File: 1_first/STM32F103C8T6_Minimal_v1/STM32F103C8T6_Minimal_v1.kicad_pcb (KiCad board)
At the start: 4 copper layers, 34 parts, among them J1 Conn_01x06, J2 USB_B_Micro, SW1 SW_SPDT, SW2 SW_Push, SW3 SW_Push, U1 AMS1117-3.3, U2 STM32F103C8Tx, U3 USBLC6-2SC6, Y1 8MHz

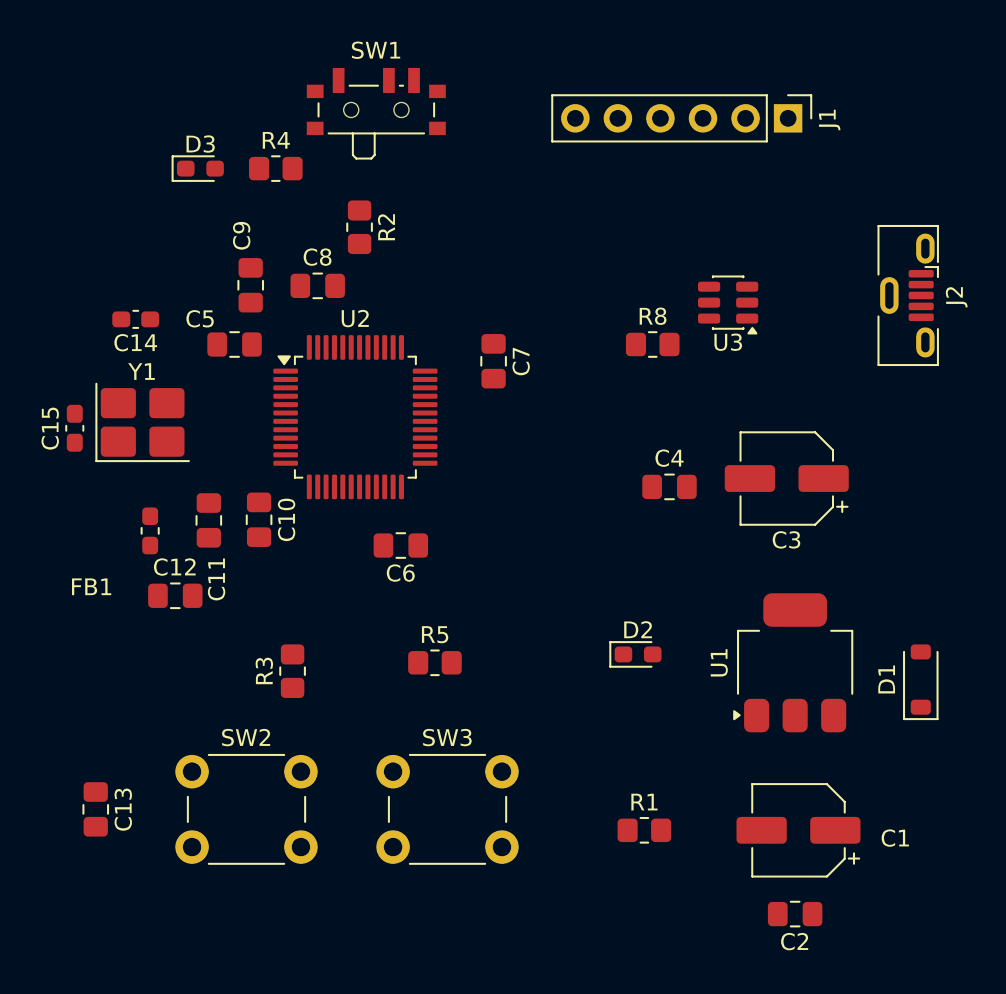
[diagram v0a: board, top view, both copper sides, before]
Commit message: Board cut
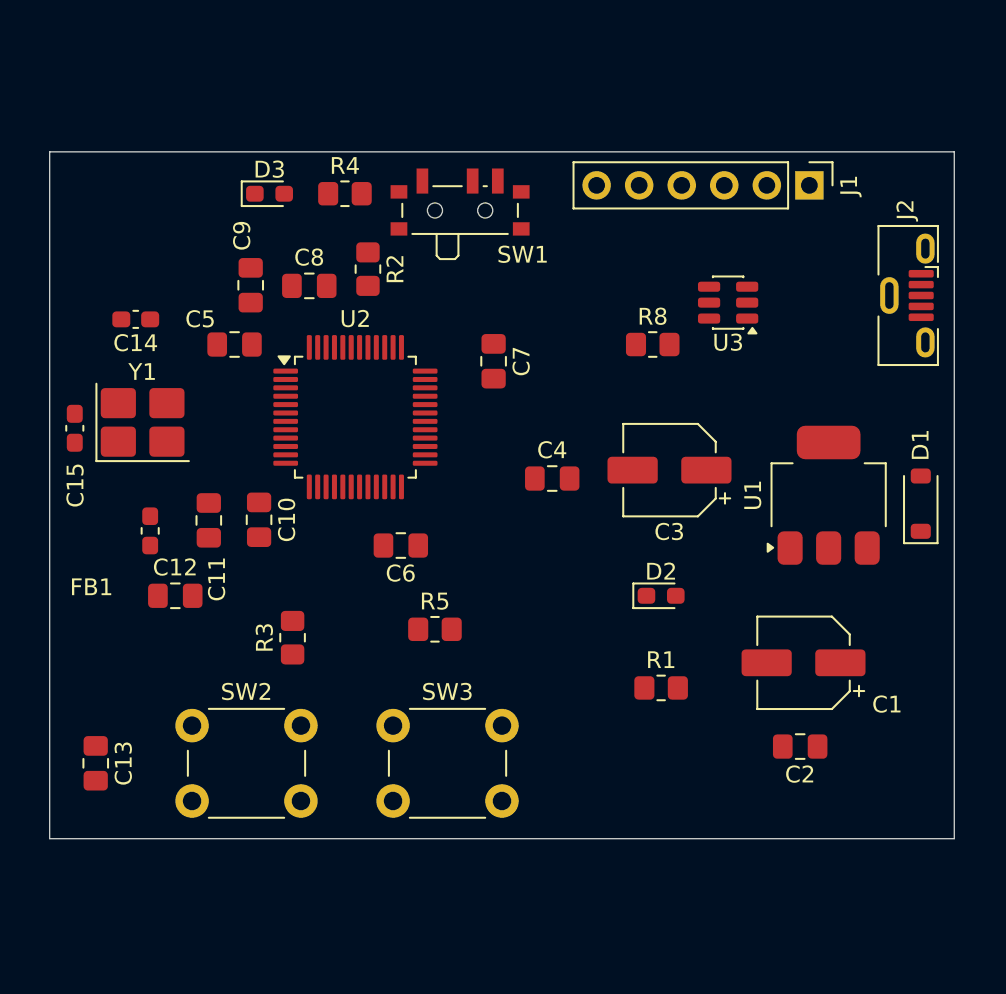
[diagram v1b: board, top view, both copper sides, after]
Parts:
- moved D1 10.5 mm to (154.0, 100.0)
- moved U1 10.2 mm to (148.5, 99.5)
- moved C1 10.0 mm to (147.0, 109.5)
- moved C2 10.0 mm to (146.8, 114.5)
- moved R1 8.56 mm to (138.5, 111.0)
- moved SW1 7.81 mm to (126.5, 82.2)
- moved C3 7.02 mm to (139.0, 98.0)
- moved C4 7.02 mm to (132.0, 98.5)
- moved D3 4.39 mm to (115.1, 81.5)
- moved R4 4.39 mm to (119.6, 81.5)
- moved J1 4.20 mm to (147.3, 81.0)
- moved D2 3.76 mm to (138.5, 105.5)
- moved C13 2.75 mm to (104.8, 115.5)
- moved SW2 2.75 mm to (110.5, 113.2)
- moved SW3 2.75 mm to (122.5, 113.2)
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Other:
- board outline added: 54 x 41 mm
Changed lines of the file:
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@@
 	(footprint "Capacitor_SMD:CP_Elec_5x5.3"
 		(layer "F.Cu")
-		(at 146.7 119.5 180)
+		(at 147 109.5 180)
 		(descr "SMD capacitor, aluminum electrolytic, Nichicon, 5.0x5.3mm")
 		(tags "capacitor electrolytic")
 		(property "Reference" "C1"
-			(at -5.8 -0.5 0)
+			(at -5 -2.5 0)
 			(layer "F.SilkS")
 			(effects
@@
 	(footprint "Connector_PinHeader_2.54mm:PinHeader_1x06_P2.54mm_Vertical"
 		(layer "F.Cu")
-		(at 146.08 77 -90)
+		(at 147.35 81 -90)
 		(descr "Through hole straight pin header, 1x06, 2.54mm pitch, single row")
 		(tags "Through hole pin header THT 1x06 2.54mm single row")
@@
 		)
 		(property "Value" "Conn_01x06"
-			(at 0 15.08 90)
+			(at 2.35 7.4 180)
 			(layer "F.Fab")
 			(effects
@@
 	(footprint "Capacitor_SMD:CP_Elec_5x5.3"
 		(layer "F.Cu")
-		(at 146 98.5 180)
+		(at 139 98 180)
 		(descr "SMD capacitor, aluminum electrolytic, Nichicon, 5.0x5.3mm")
 		(tags "capacitor electrolytic")
@@
 	(footprint "Button_Switch_THT:SW_PUSH_6mm_H5mm"
 		(layer "F.Cu")
-		(at 122.5 116)
+		(at 122.5 113.25)
 		(descr "tactile push button, 6x6mm e.g. PHAP33xx series, height=5mm")
 		(tags "tact sw push 6mm")
@@
 		)
 		(property "Value" "SW_Push"
-			(at 3.75 6.7 0)
+			(at 11.35 2.5 0)
 			(layer "F.Fab")
 			(effects
@@
 	(footprint "Button_Switch_THT:SW_PUSH_6mm_H5mm"
 		(layer "F.Cu")
-		(at 110.5 116)
+		(at 110.5 113.25)
 		(descr "tactile push button, 6x6mm e.g. PHAP33xx series, height=5mm")
 		(tags "tact sw push 6mm")
@@
 		)
 		(property "Value" "SW_Push"
-			(at 3.75 6.7 0)
+			(at -4.75 5.45 0)
 			(layer "F.Fab")
 			(effects
@@
 	(footprint "Resistor_SMD:R_0805_2012Metric_Pad1.20x1.40mm_HandSolder"
 		(layer "F.Cu")
-		(at 115.5 80)
+		(at 119.625 81.5)
 		(descr "Resistor SMD 0805 (2012 Metric), square (rectangular) end terminal, IPC-7351 nominal with elongated pad for handsoldering. (Body size source: IPC-SM-782 page 72, https://www.pcb-3d.com/wordpress/wp-content/uploads/ipc-sm-782a_amendment_1_and_2.pdf)")
 		(tags "resistor handsolder")
@@
 	(footprint "Resistor_SMD:R_0805_2012Metric_Pad1.20x1.40mm_HandSolder"
 		(layer "F.Cu")
-		(at 120.5 83.5 -90)
+		(at 121 86 -90)
 		(descr "Resistor SMD 0805 (2012 Metric), square (rectangular) end terminal, IPC-7351 nominal with elongated pad for handsoldering. (Body size source: IPC-SM-782 page 72, https://www.pcb-3d.com/wordpress/wp-content/uploads/ipc-sm-782a_amendment_1_and_2.pdf)")
 		(tags "resistor handsolder")
@@
 	(footprint "LED_SMD:LED_0603_1608Metric_Pad1.05x0.95mm_HandSolder"
 		(layer "F.Cu")
-		(at 111 80)
+		(at 115.125 81.5)
 		(descr "LED SMD 0603 (1608 Metric), square (rectangular) end terminal, IPC-7351 nominal, (Body size source: http://www.tortai-tech.com/upload/download/2011102023233369053.pdf)")
 		(tags "LED handsolder")
@@
 	(footprint "Resistor_SMD:R_0805_2012Metric_Pad1.20x1.40mm_HandSolder"
 		(layer "F.Cu")
-		(at 125 109.5)
+		(at 125 107.5)
 		(descr "Resistor SMD 0805 (2012 Metric), square (rectangular) end terminal, IPC-7351 nominal with elongated pad for handsoldering. (Body size source: IPC-SM-782 page 72, https://www.pcb-3d.com/wordpress/wp-content/uploads/ipc-sm-782a_amendment_1_and_2.pdf)")
 		(tags "resistor handsolder")
@@
 	(footprint "LED_SMD:LED_0603_1608Metric_Pad1.05x0.95mm_HandSolder"
 		(layer "F.Cu")
-		(at 137.125 109)
+		(at 138.5 105.5)
 		(descr "LED SMD 0603 (1608 Metric), square (rectangular) end terminal, IPC-7351 nominal, (Body size source: http://www.tortai-tech.com/upload/download/2011102023233369053.pdf)")
 		(tags "LED handsolder")
@@
 	(footprint "Diode_SMD:D_SOD-123"
 		(layer "F.Cu")
-		(at 154 110.5 90)
+		(at 154 100 90)
 		(descr "SOD-123")
 		(tags "SOD-123")
 		(property "Reference" "D1"
-			(at 0 -2 90)
+			(at 3.5 0 90)
 			(layer "F.SilkS")
 			(effects
@@
 		)
 		(property "Value" "D_Schottky"
-			(at 0 2.1 90)
+			(at -6.5 0 270)
 			(layer "F.Fab")
 			(effects
@@
 		)
 		(fp_text user "${REFERENCE}"
-			(at 0 -2 90)
+			(at 3.5 0 90)
 			(layer "F.Fab")
 			(effects
@@
 	(footprint "Capacitor_SMD:C_0805_2012Metric_Pad1.18x1.45mm_HandSolder"
 		(layer "F.Cu")
-		(at 118 87)
+		(at 117.5 87)
 		(descr "Capacitor SMD 0805 (2012 Metric), square (rectangular) end terminal, IPC-7351 nominal with elongated pad for handsoldering. (Body size source: IPC-SM-782 page 76, https://www.pcb-3d.com/wordpress/wp-content/uploads/ipc-sm-782a_amendment_1_and_2.pdf, https://docs.google.com/spreadsheets/d/1BsfQQcO9C6DZCsRaXUlFlo91Tg2WpOkGARC1WS5S8t0/edit?usp=sharing)")
 		(tags "capacitor handsolder")
@@
 	(footprint "Package_TO_SOT_SMD:SOT-223-3_TabPin2"
 		(layer "F.Cu")
-		(at 146.5 109.5 90)
+		(at 148.5 99.5 90)
 		(descr "module CMS SOT223 4 pins")
 		(tags "CMS SOT")
@@
 		)
 		(property "Value" "AMS1117-3.3"
-			(at 0 4.5 90)
+			(at 5.5 0 180)
 			(layer "F.Fab")
 			(effects
@@
 	(footprint "Button_Switch_SMD:SW_SPDT_PCM12"
 		(layer "F.Cu")
-		(at 121.5 76.17)
+		(at 126.5 82.17)
 		(descr "Ultraminiature Surface Mount Slide Switch, right-angle, https://www.ckswitches.com/media/1424/pcm.pdf")
 		(property "Reference" "SW1"
-			(at 0 -3.2 0)
+			(at 3.75 2.98 0)
 			(layer "F.SilkS")
 			(effects
@@
 		)
 		(fp_text user "${REFERENCE}"
-			(at 0 -3.2 0)
+			(at 3.75 2.98 0)
 			(layer "F.Fab")
 			(effects
@@
 	(footprint "Capacitor_SMD:C_0805_2012Metric_Pad1.18x1.45mm_HandSolder"
 		(layer "F.Cu")
-		(at 104.75 118.25 -90)
+		(at 104.75 115.5 -90)
 		(descr "Capacitor SMD 0805 (2012 Metric), square (rectangular) end terminal, IPC-7351 nominal with elongated pad for handsoldering. (Body size source: IPC-SM-782 page 76, https://www.pcb-3d.com/wordpress/wp-content/uploads/ipc-sm-782a_amendment_1_and_2.pdf, https://docs.google.com/spreadsheets/d/1BsfQQcO9C6DZCsRaXUlFlo91Tg2WpOkGARC1WS5S8t0/edit?usp=sharing)")
 		(tags "capacitor handsolder")
@@
 	(footprint "Capacitor_SMD:C_0805_2012Metric_Pad1.18x1.45mm_HandSolder"
 		(layer "F.Cu")
-		(at 146.5 124.5 180)
+		(at 146.8 114.5 180)
 		(descr "Capacitor SMD 0805 (2012 Metric), square (rectangular) end terminal, IPC-7351 nominal with elongated pad for handsoldering. (Body size source: IPC-SM-782 page 76, https://www.pcb-3d.com/wordpress/wp-content/uploads/ipc-sm-782a_amendment_1_and_2.pdf, https://docs.google.com/spreadsheets/d/1BsfQQcO9C6DZCsRaXUlFlo91Tg2WpOkGARC1WS5S8t0/edit?usp=sharing)")
 		(tags "capacitor handsolder")
@@
 	(footprint "Resistor_SMD:R_0805_2012Metric_Pad1.20x1.40mm_HandSolder"
 		(layer "F.Cu")
-		(at 116.5 110 90)
+		(at 116.5 108 90)
 		(descr "Resistor SMD 0805 (2012 Metric), square (rectangular) end terminal, IPC-7351 nominal with elongated pad for handsoldering. (Body size source: IPC-SM-782 page 72, https://www.pcb-3d.com/wordpress/wp-content/uploads/ipc-sm-782a_amendment_1_and_2.pdf)")
 		(tags "resistor handsolder")
@@
 		(tags "capacitor handsolder")
 		(property "Reference" "C15"
-			(at 0 -1.43 90)
+			(at -3.4 0.05 90)
 			(layer "F.SilkS")
 			(effects
@@
 	(footprint "Capacitor_SMD:C_0805_2012Metric_Pad1.18x1.45mm_HandSolder"
 		(layer "F.Cu")
-		(at 139 99)
+		(at 132 98.5)
 		(descr "Capacitor SMD 0805 (2012 Metric), square (rectangular) end terminal, IPC-7351 nominal with elongated pad for handsoldering. (Body size source: IPC-SM-782 page 76, https://www.pcb-3d.com/wordpress/wp-content/uploads/ipc-sm-782a_amendment_1_and_2.pdf, https://docs.google.com/spreadsheets/d/1BsfQQcO9C6DZCsRaXUlFlo91Tg2WpOkGARC1WS5S8t0/edit?usp=sharing)")
 		(tags "capacitor handsolder")
@@
 	(footprint "Resistor_SMD:R_0805_2012Metric_Pad1.20x1.40mm_HandSolder"
 		(layer "F.Cu")
-		(at 137.5 119.5)
+		(at 138.5 111)
 		(descr "Resistor SMD 0805 (2012 Metric), square (rectangular) end terminal, IPC-7351 nominal with elongated pad for handsoldering. (Body size source: IPC-SM-782 page 72, https://www.pcb-3d.com/wordpress/wp-content/uploads/ipc-sm-782a_amendment_1_and_2.pdf)")
 		(tags "resistor handsolder")
@@
 		(tags "Micro-USB SMD Typ-B Vertical")
 		(property "Reference" "J2"
-			(at 0 -2.85 90)
+			(at -5.125 0.1 90)
 			(layer "F.SilkS")
 			(effects
@@
 		)
 	)
+	(gr_line
+		(start 102 120)
+		(end 102 79)
+		(stroke
+			(width 0.05)
+			(type default)
+		)
+		(layer "Edge.Cuts")
+	)
+	(gr_line
+		(start 102 120)
+		(end 156 120)
+		(stroke
+			(width 0.05)
+			(type default)
+		)
+		(layer "Edge.Cuts")
+	)
+	(gr_line
+		(start 156 79)
+		(end 102 79)
+		(stroke
+			(width 0.05)
+			(type default)
+		)
+		(layer "Edge.Cuts")
+	)
+	(gr_line
+		(start 156 120)
+		(end 156 79)
+		(stroke
+			(width 0.05)
+			(type default)
+		)
+		(layer "Edge.Cuts")
+	)
 	(embedded_fonts no)
